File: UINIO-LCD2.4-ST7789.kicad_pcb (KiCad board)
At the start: 2 copper layers, 35 parts, among them CON1 FFC_8Pin_0.5mm, J1 Conn_01x08_Male, Q1 S8050, U1 ME6211C33M5G-N, U2 AMS1117, U3 XC6206P332MR, U4 CON_10Pin

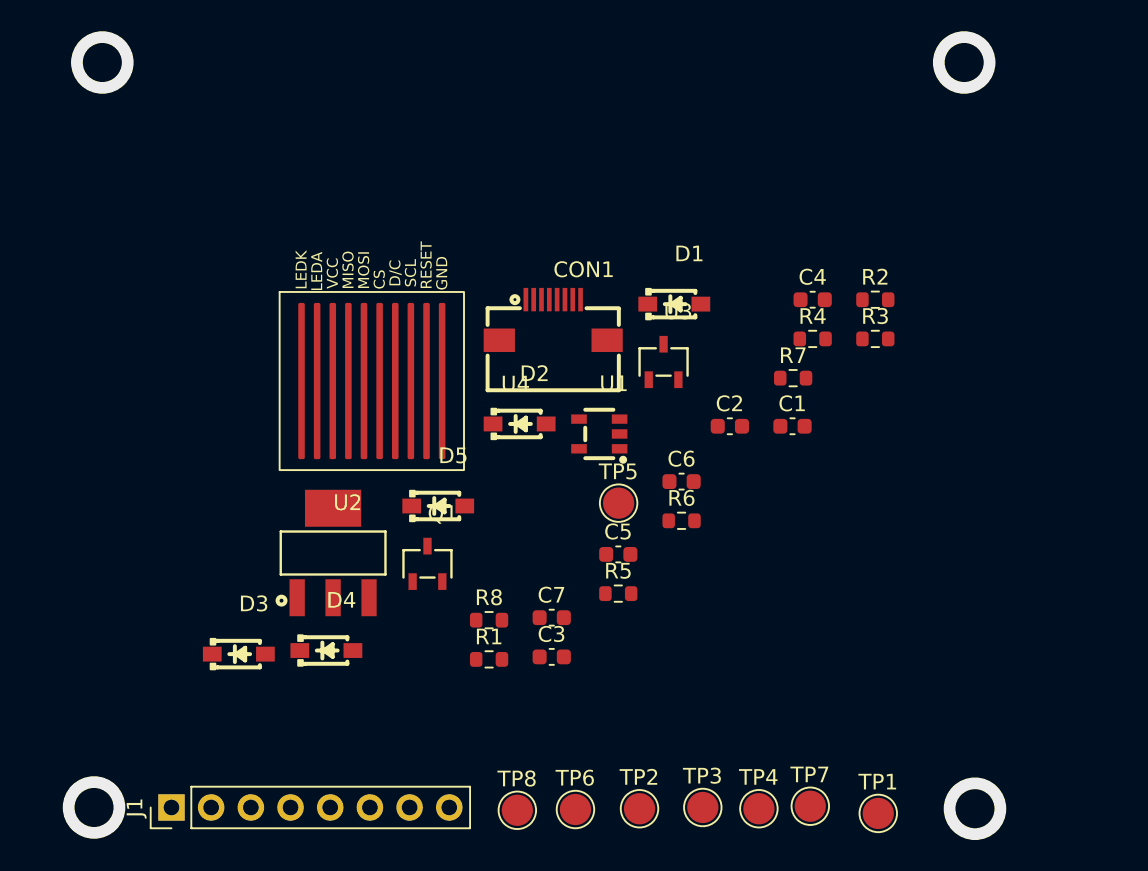
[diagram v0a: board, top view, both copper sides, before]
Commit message: start drawing PCB.
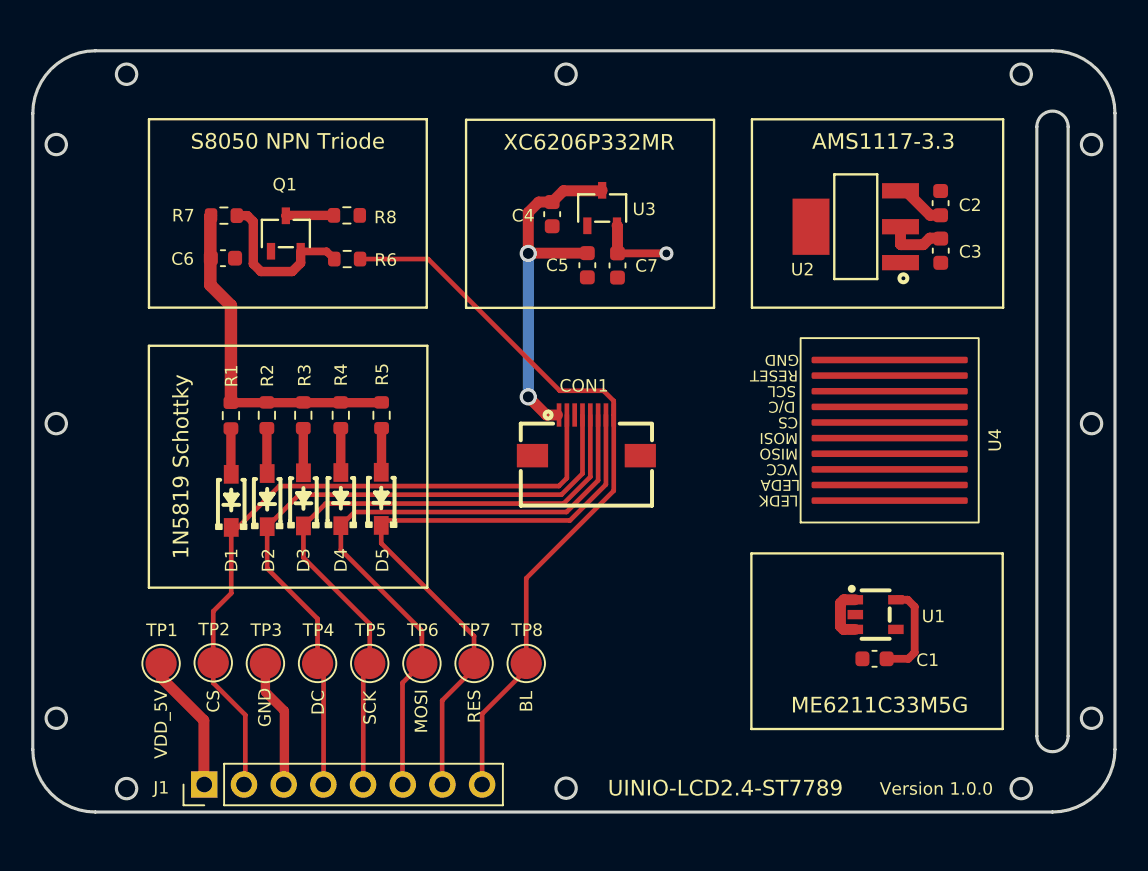
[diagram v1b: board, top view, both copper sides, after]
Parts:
- TP2: value CS -> GND
- TP3: value GND -> CS
- TP7: value CS -> RES
- moved TP1 46.9 mm to (135.6, 120.6)
- moved R2 39.6 mm to (142.4, 104.7), turned to 90 degrees
- moved U2 39.4 mm to (180.1, 92.6), turned to 90 degrees
- moved R7 37.9 mm to (139.6, 91.9)
- moved R3 36.9 mm to (144.7, 104.7), turned to 90 degrees
- moved C3 36.0 mm to (185.5, 94.1), turned to -90 degrees
- moved U4 33.6 mm to (182.5, 105.6), turned to 90 degrees
- moved C6 32.6 mm to (139.6, 94.6)
- moved D1 31.0 mm to (140.1, 110.2), turned to 90 degrees
- moved R4 30.6 mm to (147.1, 104.7), turned to 90 degrees
- moved TP4 29.7 mm to (145.6, 120.6)
- moved TP3 29.5 mm to (142.3, 120.6)
- moved TP2 28.8 mm to (138.9, 120.5)
- moved R8 27.5 mm to (147.5, 91.9)
- moved R6 27.2 mm to (147.5, 94.7), turned to 180 degrees
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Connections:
- CON1 pad 1: GND -> /VDD_5V
- CON1 pad 2: /VCC -> Net-(CON1-Pad2)
- CON1 pad 3: Net-(CON1-Pad3) -> GND
- D1 pad 1: Net-(CON1-Pad3) -> Net-(CON1-Pad2)
- D1 pad 2: GND -> /CS
- D5 pad 2: /CS -> /RES
- J1 pad 1: GND -> /VDD_5V
- J1 pad 2: /VCC -> Net-(CON1-Pad2)
- J1 pad 3: Net-(CON1-Pad3) -> GND
- R1 pad 1: GND -> /CS
- R5 pad 1: /CS -> /RES
- TP1 pad 1: GND -> /VDD_5V
- TP2 pad 1: /VCC -> Net-(CON1-Pad2)
- TP3 pad 1: Net-(CON1-Pad3) -> GND
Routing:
- net /BL: track 0.00 -> 48.0 mm
- net Net-(CON1-Pad2): track 0.00 -> 44.6 mm
- net Net-(CON1-Pad4): track 0.00 -> 43.3 mm
- net Net-(CON1-Pad5): track 0.00 -> 42.1 mm
- net Net-(CON1-Pad6): track 0.00 -> 41.1 mm
- net Net-(CON1-Pad7): track 0.00 -> 39.8 mm
- net /VDD_5V: track 0.00 -> 38.9 mm, vias 0 -> 2
- net /VDD_3.3V: track 0.00 -> 37.3 mm, vias 0 -> 1
- net Net-(Q1-Pad2): track 0.00 -> 10.5 mm
- net GND: track 0.00 -> 8.27 mm, vias 4 -> 0
- net Net-(Q1-Pad3): track 0.00 -> 3.09 mm
- net /CS: track 0.00 -> 2.94 mm
- net /DC: track 0.00 -> 2.91 mm
- net /SCK: track 0.00 -> 2.86 mm
- net /MOSI: track 0.00 -> 2.84 mm
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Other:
- board outline added: 69.3 x 48.7 mm
- board text added: "1N5819 Schottky"
- board text added: "AMS1117-3.3"
- board text added: "BL"
- board text added: "CS"
- board text added: "DC"
- board text added: "GND"
- board text added: "ME6211C33M5G"
- board text added: "MOSI"
- board text added: "RES"
- board text added: "S8050 NPN Triode"
- board text added: "SCK"
- board text added: "UINIO-LCD2.4-ST7789"
- board text added: "VDD_5V"
- board text added: "Version 1.0.0"
- board text added: "XC6206P332MR"
